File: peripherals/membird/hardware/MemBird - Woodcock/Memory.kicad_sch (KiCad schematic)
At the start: 8 parts, among them U16 AS6C8016, U17 AS6C8016, U18 AS6C8016, U19 AS6C8016

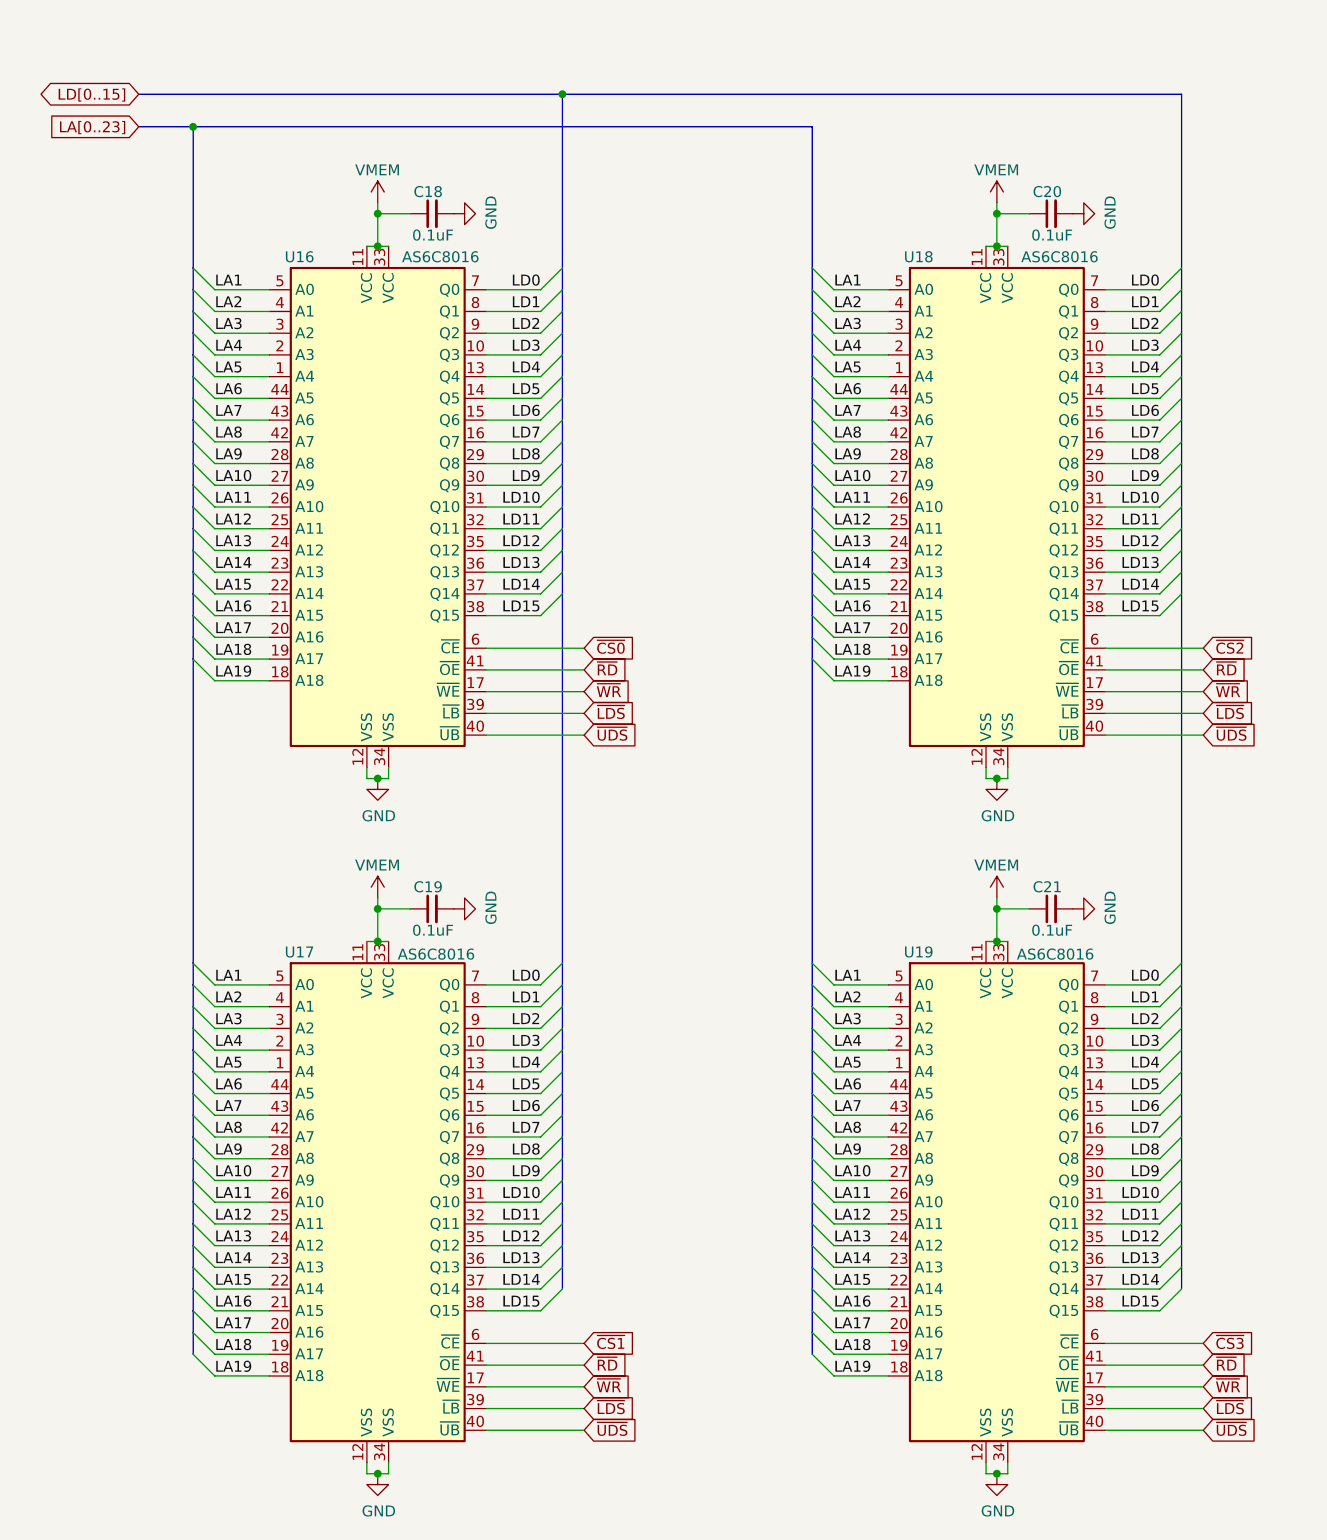
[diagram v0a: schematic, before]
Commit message: k30p-VME rev.1, MemBird Woodcock rev.1, and frontpanels
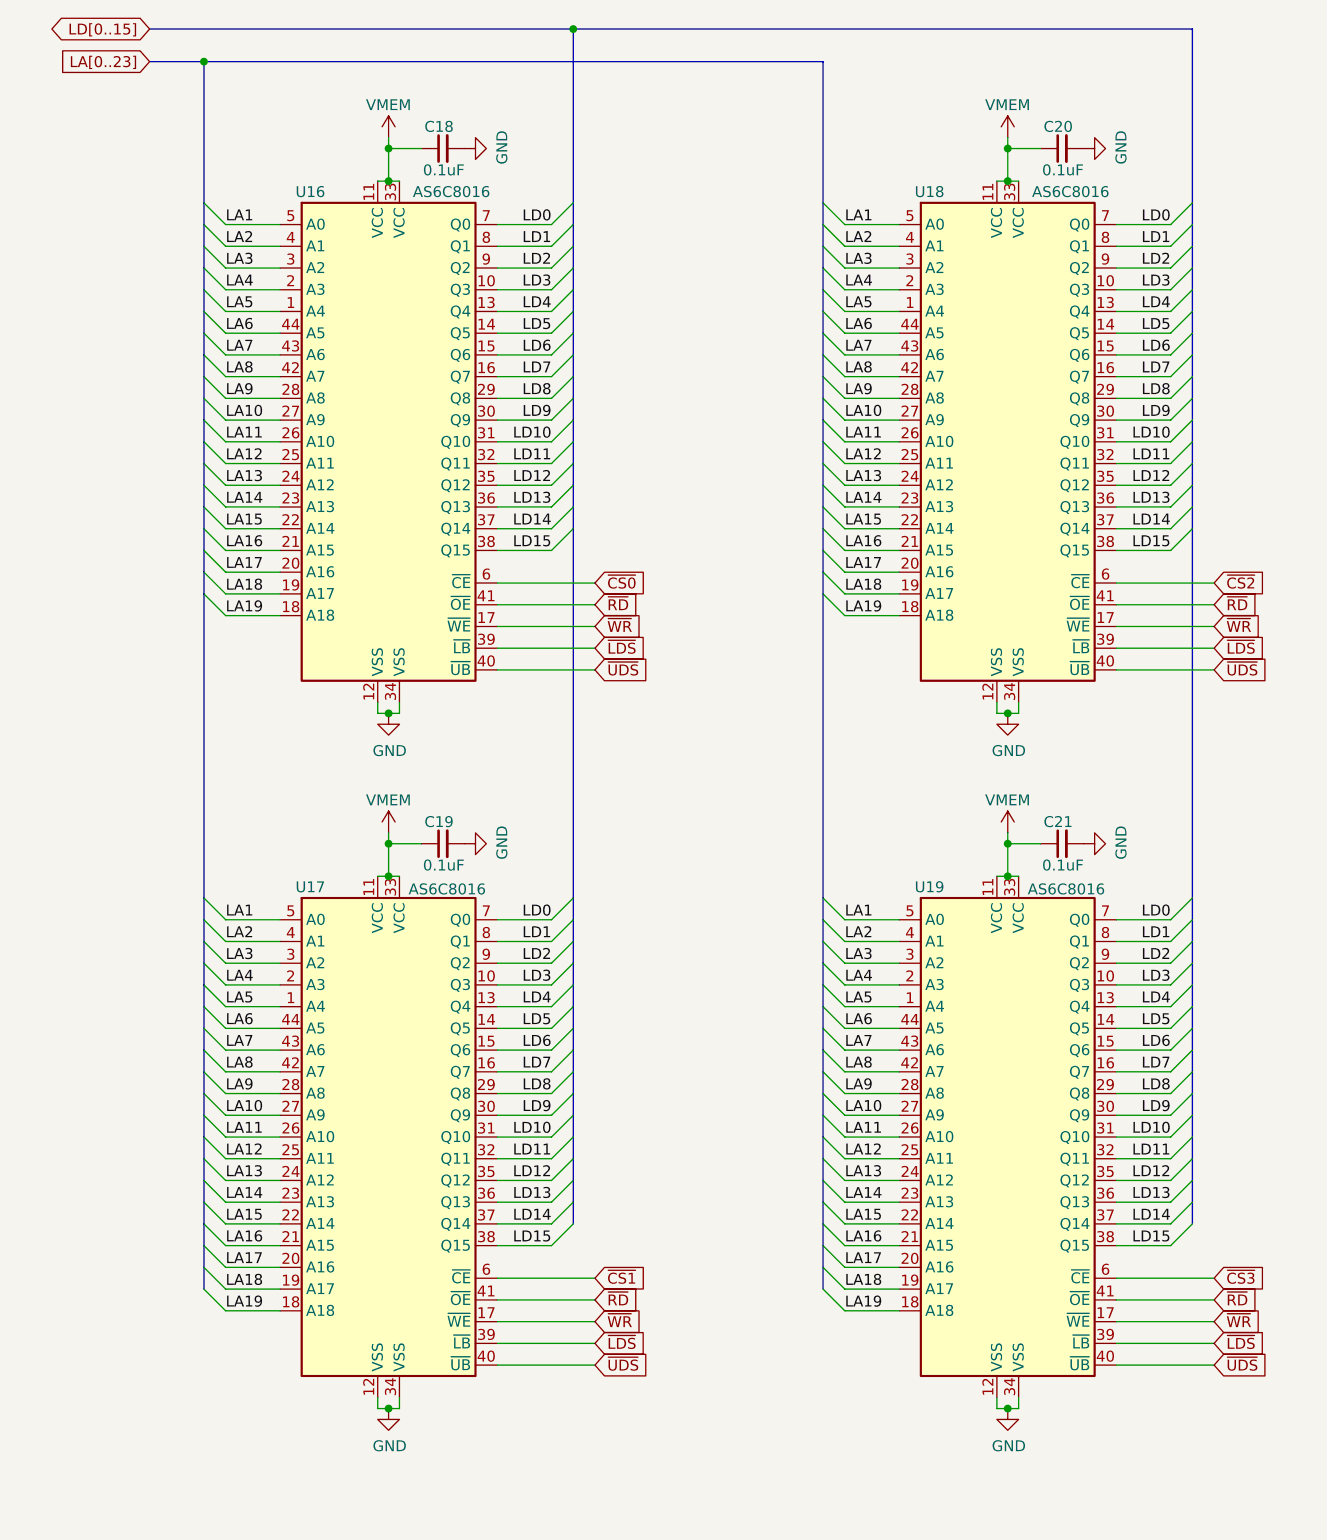
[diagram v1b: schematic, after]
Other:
- moved on the sheet: C18, C19, C20, C21, U16, U17, U18, U19
